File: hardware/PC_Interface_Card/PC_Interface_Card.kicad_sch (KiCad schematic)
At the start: 87 parts, among them J1 GSB1C41110SSHR, J2 DM3BT-DSF-PEJS, J3 GHR-11V-S, J4 BM11B-GHS-TBT, J5 GHR-11V-S, SW1 CherryMX, SW2 CherryMX, SW3 CherryMX, SW4 CherryMX, SW5 CherryMX, SW6 TL1240YQ2JBLK, SW7 TL1240YQ2JBLK, SW8 TL1240YQ2JBLK, U1 USBLC6-2SC6, U2 TLV1117LV33DCYR, U3 MB85RS4MTYPN-GS-AWEWE1, U4 ESP32-S3-WROOM-1

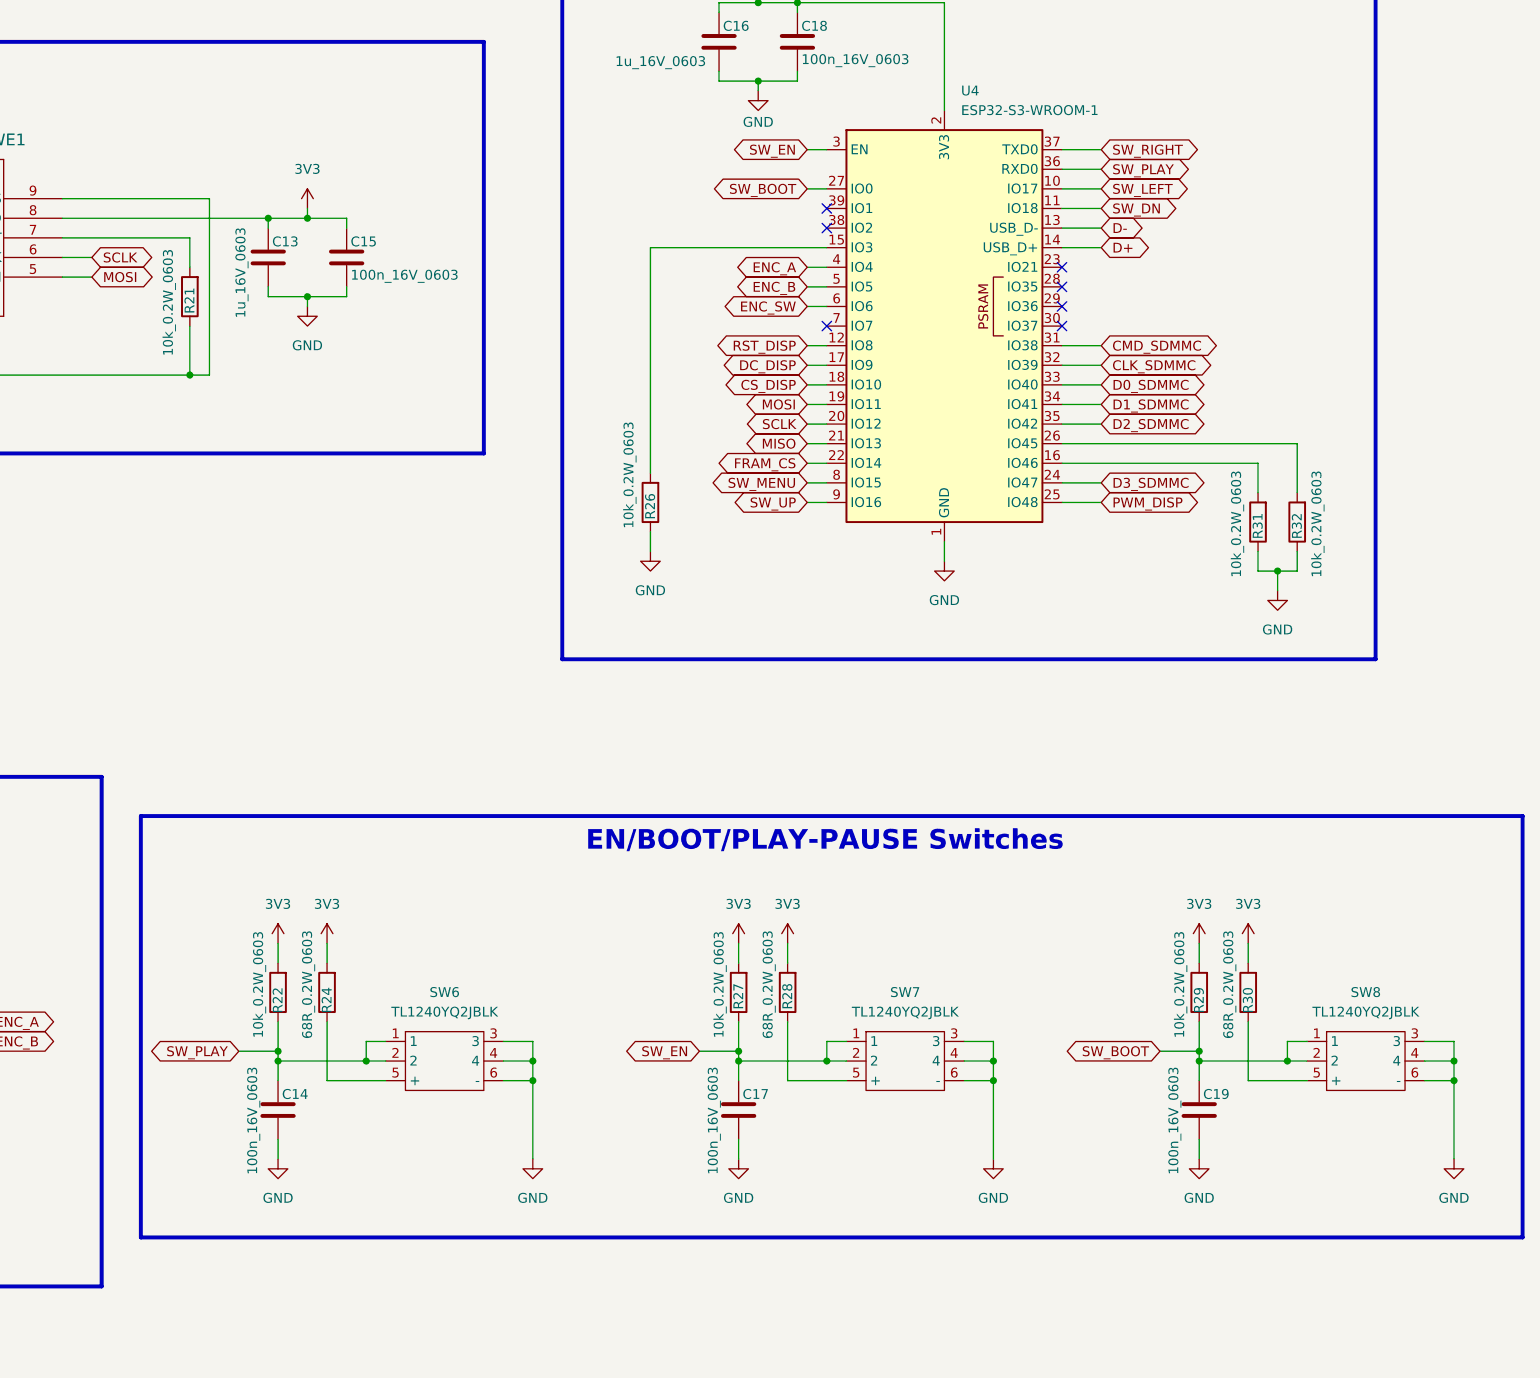
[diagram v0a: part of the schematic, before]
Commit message: layout changes
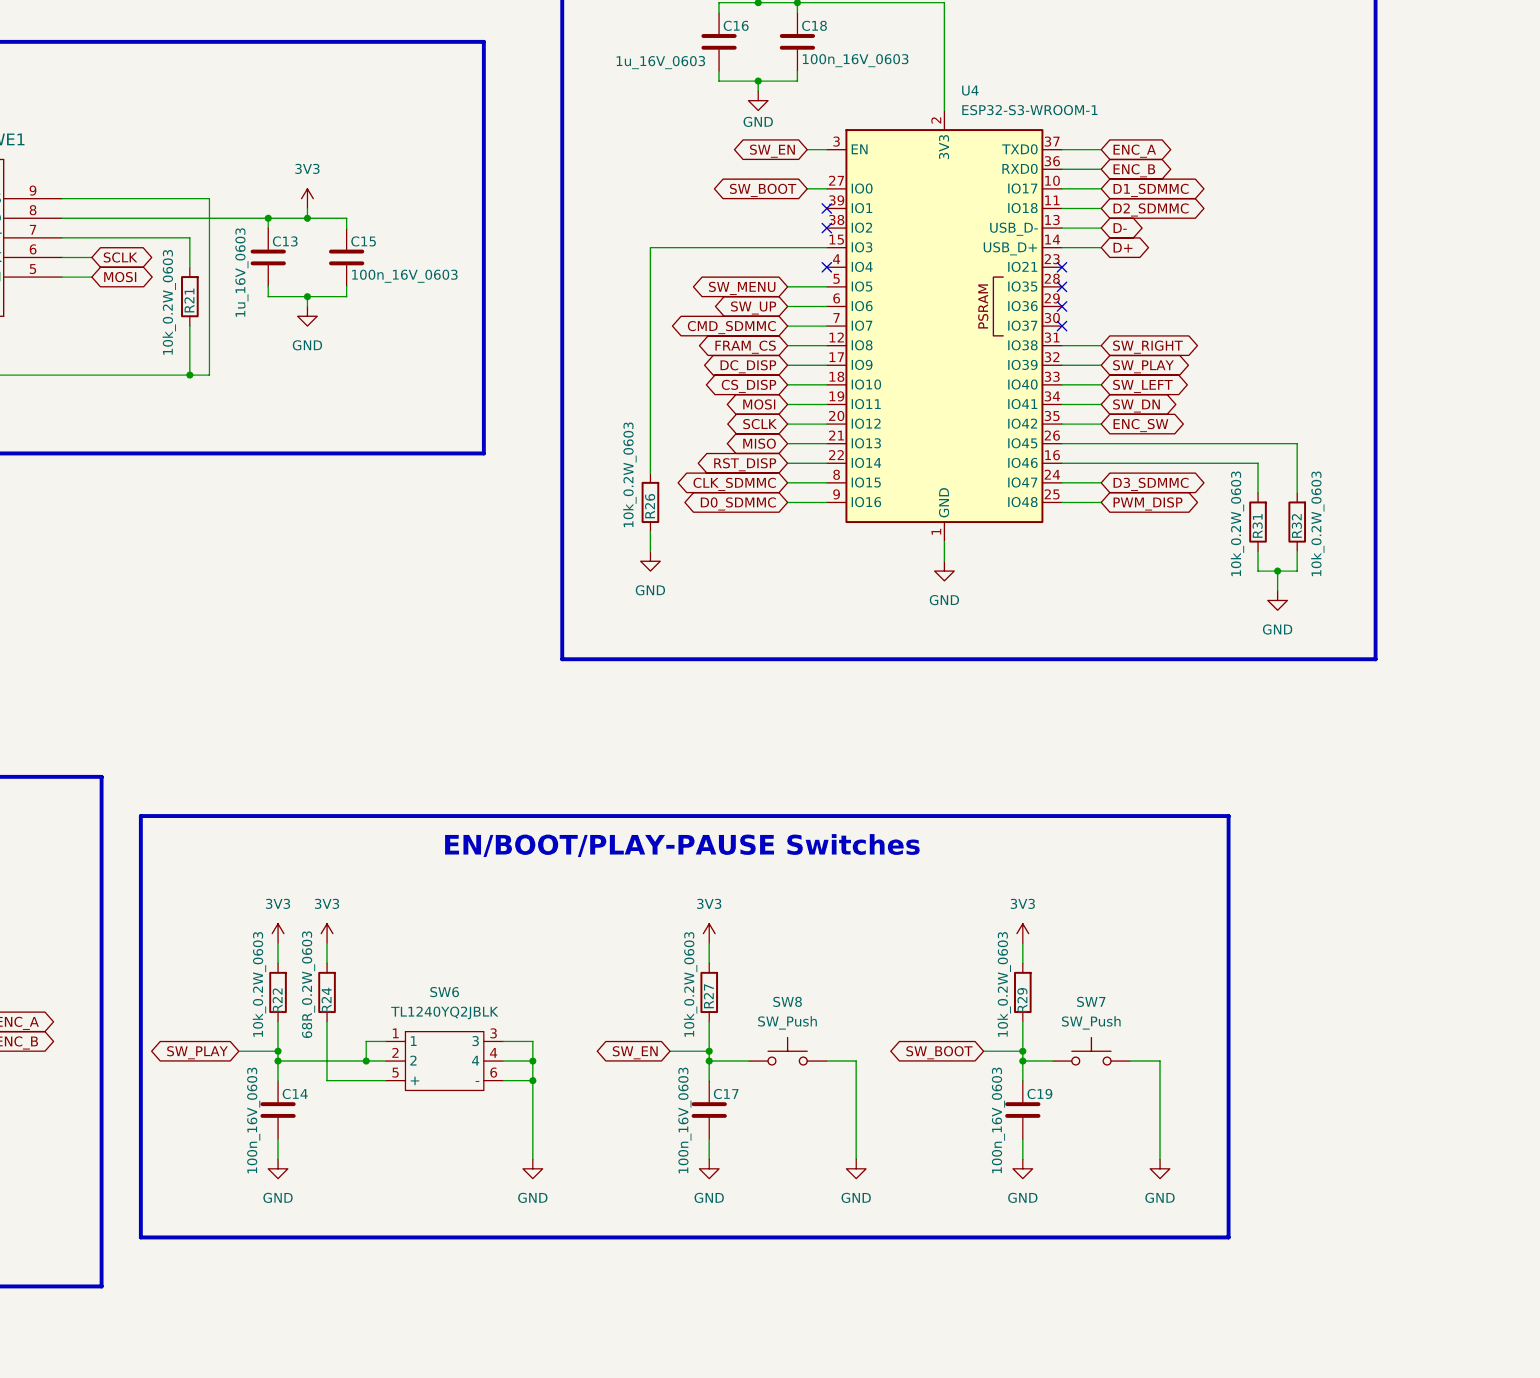
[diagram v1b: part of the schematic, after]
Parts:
- removed R28, R30: 68R_0.2W_0603, Resistor_SMD:R_0603_1608Metric, symbol Device:R
- removed SW7, SW8: TL1240YQ2JBLK, Footprint:TL1240YQ, symbol Custom_Switch_LED:TL1240YQ2JBLK
- added SW7, SW8: SW_Push, Button_Switch_THT:SW_PUSH_6mm, symbol Switch:SW_Push
- U4: footprint RF_Module:ESP32-S3-WROOM-1 -> RF_Module:ESP32-S3-WROOM-1U
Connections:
- net CLK_SDMMC: now also U4.8 (IO15); no longer U4.32 (IO39)
- net CMD_SDMMC: now also U4.7 (IO7); no longer U4.31 (IO38)
- net D0_SDMMC: now also U4.9 (IO16); no longer U4.33 (IO40)
- net D1_SDMMC: now also U4.10 (IO17); no longer U4.34 (IO41)
- net D2_SDMMC: now also U4.11 (IO18); no longer U4.35 (IO42)
- net ENC_A: now also U4.37 (TXD0); no longer U4.4 (IO4)
- net ENC_B: now also U4.36 (RXD0); no longer U4.5 (IO5)
- net ENC_SW: now also U4.35 (IO42); no longer U4.6 (IO6)
- net FRAM_CS: now also U4.12 (IO8); no longer U4.22 (IO14)
- net GND: now also SW7.2, SW8.2
- net RST_DISP: now also U4.22 (IO14); no longer U4.12 (IO8)
- net SW_BOOT: now also SW7.1
- net SW_DN: now also U4.34 (IO41); no longer U4.11 (IO18)
- net SW_EN: now also SW8.1
- net SW_LEFT: now also U4.33 (IO40); no longer U4.10 (IO17)
- net SW_MENU: now also U4.5 (IO5); no longer U4.8 (IO15)
- net SW_PLAY: now also U4.32 (IO39); no longer U4.36 (RXD0)
- net SW_RIGHT: now also U4.31 (IO38); no longer U4.37 (TXD0)
- net SW_UP: now also U4.6 (IO6); no longer U4.9 (IO16)
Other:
- moved on the sheet: C17, C19, R27, R29
